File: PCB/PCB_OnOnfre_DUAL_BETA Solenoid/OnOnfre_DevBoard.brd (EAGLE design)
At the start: 44.4 x 47.7 mm, 25 parts, among them J3Y S8050, J7 8p, U2 esp12

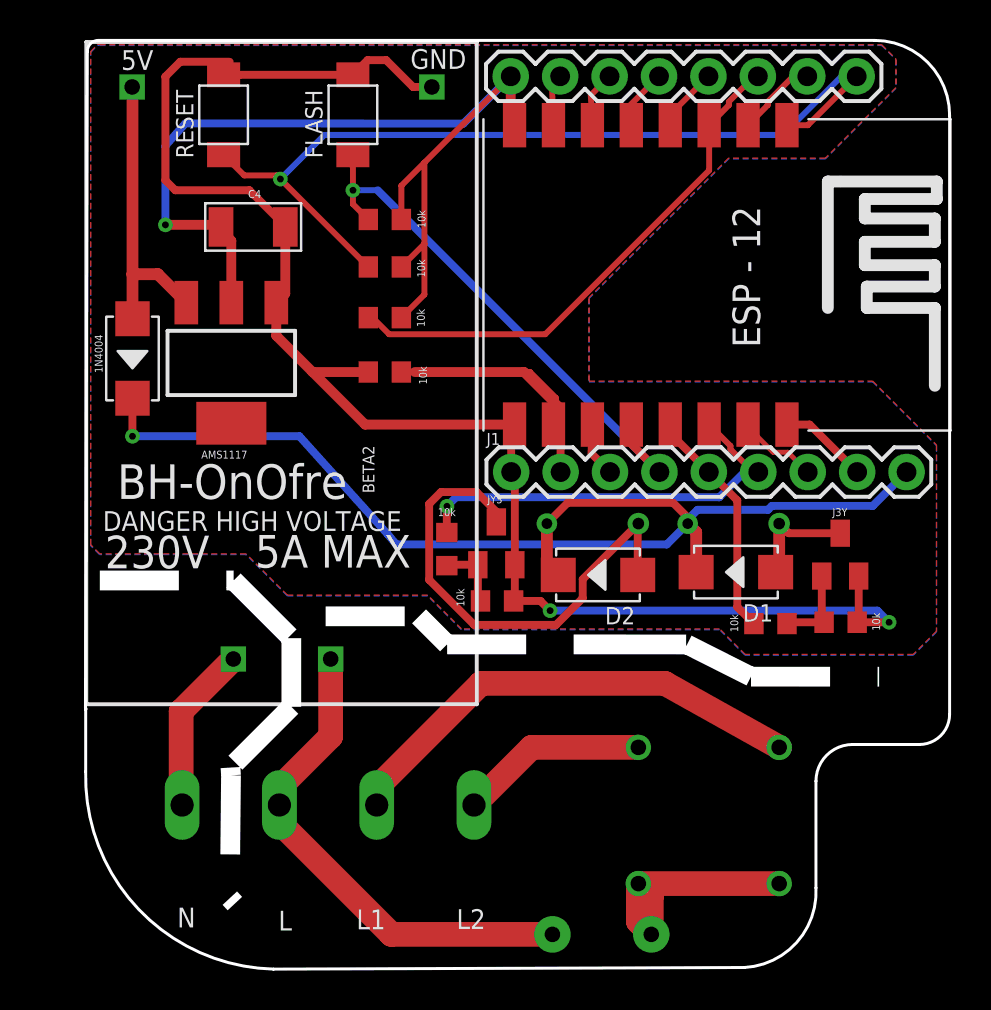
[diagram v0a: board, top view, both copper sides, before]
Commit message: 10A
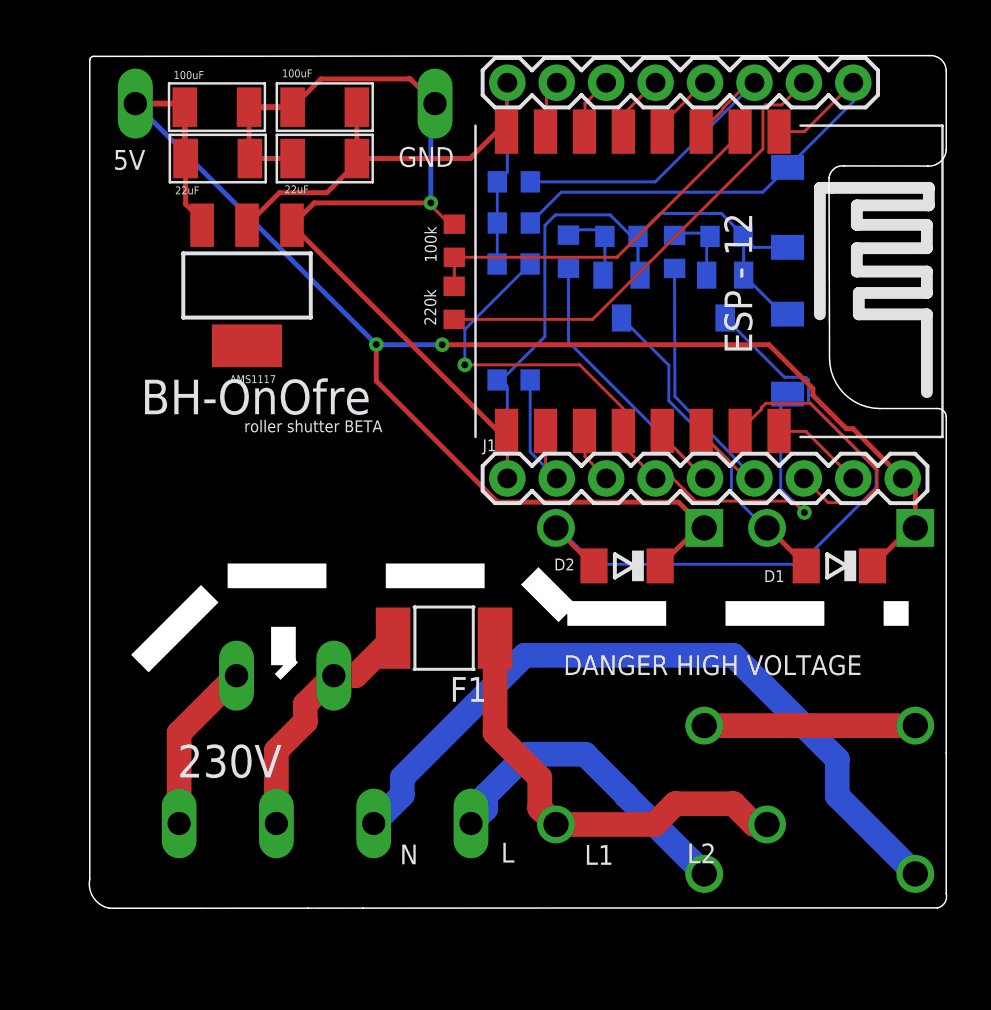
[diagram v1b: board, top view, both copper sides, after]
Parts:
- removed D3: 1N4004, Seeed-Diode:DO-214AC
- removed U$2: HKLPM01, HKLPM01:HKLPM01
- removed U$3: HF46F, HF46F:HF46F
- added C1, C2: 22uF, Seeed-Capacitor:C1206
- added C3: 100uF, Seeed-Capacitor:C1206
- added K1, K2: G5Q-1-DC12, G5Q-1-DC12:RELAY_G5Q-1-DC12
- added R6: 220k, resistor:R0603
- added R7: 100k, resistor:R0603
- C4: value 100NF -> 100uF
- D1, D2: value 1N4007 -> 1N4148; device Seeed-Diode:DO-214AC -> diode:SOD80C
- F1: value FUSE -> 1812L010; device SparkFun-Fuses:PTH -> polyfuse-smd_10:1812L
- J1: value (none) -> 9PIN 2.54MM
- U$1: value HF46F -> HLK-PM01; device HF46F:HF46F -> HLK-PM01:HLK-PM01
- moved RESET 29.4 mm to (36.5, 38.6), flipped to the bottom, turned to 270 degrees
- moved FLASH 25.5 mm to (36.5, 31.0), flipped to the bottom
- moved R3 22.8 mm to (28.0, 37.1), flipped to the bottom, turned to 0 degrees
- moved R2 22.1 mm to (33.4, 37.1), flipped to the bottom, turned to 0 degrees
- moved R4 21.7 mm to (25.3, 36.3), flipped to the bottom, turned to 90 degrees
- moved U$1 20.5 mm to (10.7, 29.2), turned to 90 degrees
- moved R1 19.2 mm to (30.7, 36.3), flipped to the bottom, turned to 90 degrees
- moved J3Y 17.4 mm to (28.0, 34.0), flipped to the bottom, turned to 180 degrees
- moved JY3 17.3 mm to (33.3, 34.0), flipped to the bottom, turned to 180 degrees
- moved F1 17.2 mm to (18.9, 16.4), flipped to the top
- moved R9 9.62 mm to (22.5, 39.9), flipped to the bottom
- moved C4 7.17 mm to (12.8, 43.7), turned to 180 degrees
- moved R8 7.01 mm to (22.5, 35.7), flipped to the bottom
- moved R10 7.00 mm to (22.5, 37.8), flipped to the bottom
- moved R11 6.63 mm to (22.5, 29.7), flipped to the bottom, turned to 0 degrees
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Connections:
- removed net 5V: D1.2, D2.2, D3.2, J1.9, U$1.C1, U$3.C1
- removed net LINE_IN: U$2.P$2, X1.1
- removed net NEUTRAL_IN_FUSED: F1.P$2, U$1.L1, U$3.L1
- removed net NEUTRAL_ONE_OUT: U$1.L2, X1.3
- removed net NEUTRAL_TWO_OUT: U$3.L2, X1.4
- new net A0: J7.7, R6.2
- new net COM: K1.2, K2.2
- new net LINE_DOWN_OUT: K2.3, X1.4
- new net LINE_FUSED: F1.1, K1.4, K2.4
- new net LINE_L: F1.2, U$1.1, X1.2
- new net LINE_UP_OUT: K1.3, X1.3
- net 3V3: now also C1.1
- net ADC: now also R6.1, R7.2; no longer J7.7
- net GND: now also C1.2, C2.2, C3.2, R7.1, U$1.3; no longer U$2.P$3
- net N$1: now also D1.A, K1.5; no longer D1.1, U$1.C2
- net N$9: now also D2.A, K2.5; no longer D2.1, U$3.C2
- net NEUTRAL_IN: now also U$1.2, X1.1; no longer F1.P$1, U$2.P$1, X1.2
- net VCC: now also C2.1, C3.1, D1.C, D2.C, J1.9, K1.1, K2.1, U$1.4; no longer D3.1, U$2.P$4
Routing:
- net VCC: track 15.3 -> 88.0 mm, vias 0 -> 2
- net 5V: track 59.7 -> 0.00 mm, vias 1 -> 0
- net LINE_UP_OUT: track 0.00 -> 37.7 mm
- net NEUTRAL_ONE_OUT: track 24.7 -> 0.00 mm
- net A0: track 0.00 -> 24.3 mm
- net LINE_FUSED: track 0.00 -> 22.6 mm
- net 3V3: track 52.8 -> 31.5 mm, vias 1 -> 0
- net RESET: track 46.2 -> 25.0 mm, vias 1 -> 0
- net NEUTRAL_IN: track 25.9 -> 8.82 mm
- net LINE_DOWN_OUT: track 0.00 -> 16.4 mm
- net ADC: track 4.19 -> 18.9 mm
- net NEUTRAL_IN_FUSED: track 13.0 -> 0.00 mm
- net LINE_L: track 0.00 -> 12.7 mm
- net N$1: track 5.91 -> 16.8 mm
- net COM: track 0.00 -> 10.8 mm
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- removed copper zone on layer 1, net GND
- removed copper zone on layer 16, net GND
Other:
- board size 44.4 x 47.7 mm -> 44.1 x 43.8 mm
- board text added: "roller shutter BETA"
- board text removed: "5A MAX"
- board text removed: "BETA2"
